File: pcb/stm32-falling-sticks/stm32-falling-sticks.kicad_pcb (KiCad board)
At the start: 2 copper layers, 112 x 87 mm, 75 parts, among them J1 MAG_01-05_OUT, J11 BUZ_OUT, J12 Barrel_Jack_MountingPin, J2 HAL_01-05_IN, J3 LCD_OUT, J4 MAG_06-10_OUT, J5 HAL_06-10_IN, J6 START_IN, J7 POT_IN, J8 MP1584EN, J9 Screw_Terminal_01x02, Q1 AO3400A, Q10 AO3400A, Q11 AO3400A, Q2 AO3400A, Q3 AO3400A, Q4 AO3400A, Q5 AO3400A, Q6 AO3400A, Q7 AO3400A, Q8 AO3400A, Q9 AO3400A, U1 YAAJ_BluePill_Part_Like_SWD_B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

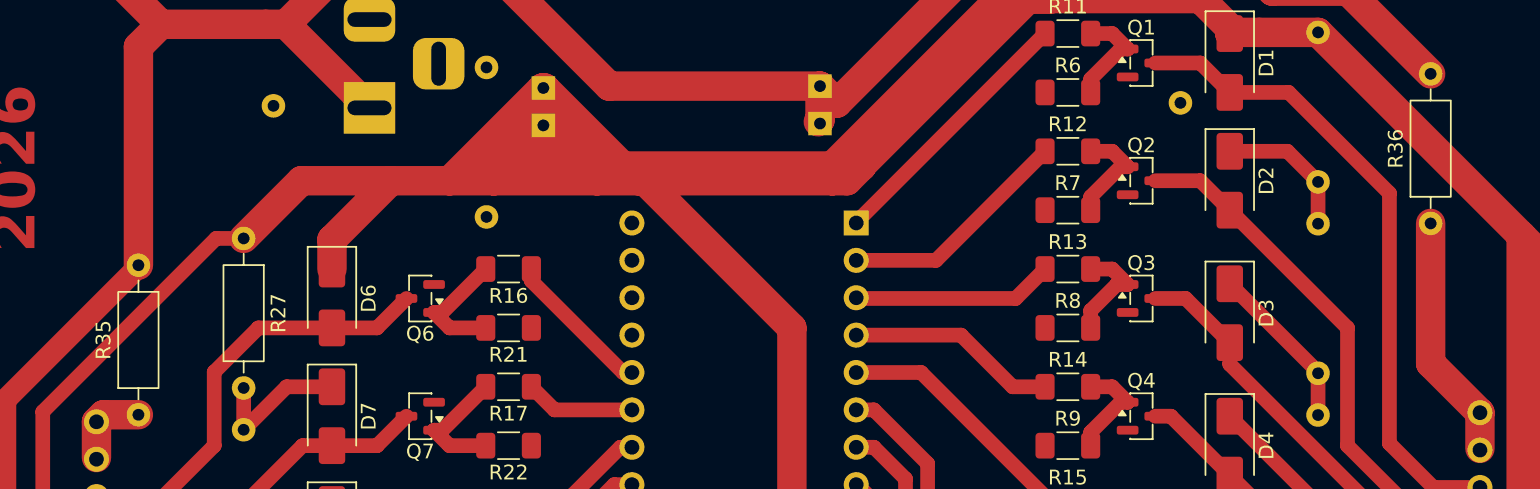
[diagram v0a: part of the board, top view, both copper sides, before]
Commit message: fix(jumper_fixes): jumper fixes
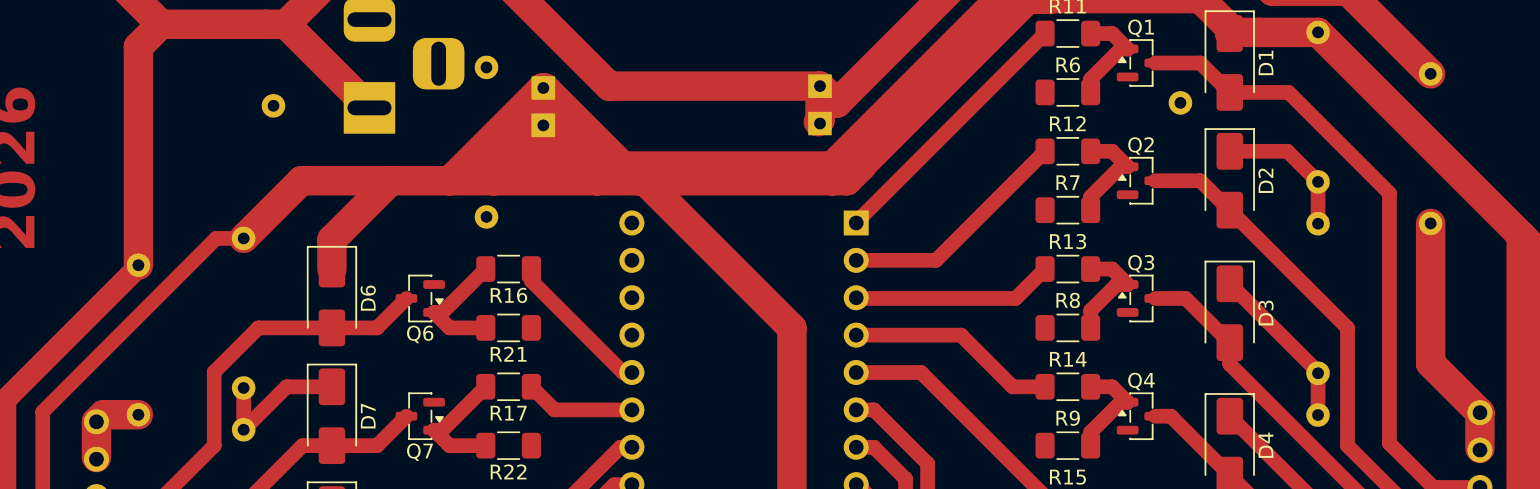
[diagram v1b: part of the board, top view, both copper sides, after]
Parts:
- R27, R35, R36: moved to B.Cu
